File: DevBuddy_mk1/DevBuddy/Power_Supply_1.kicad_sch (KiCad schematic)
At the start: 1 part, among them U5 TPS54331DDAR

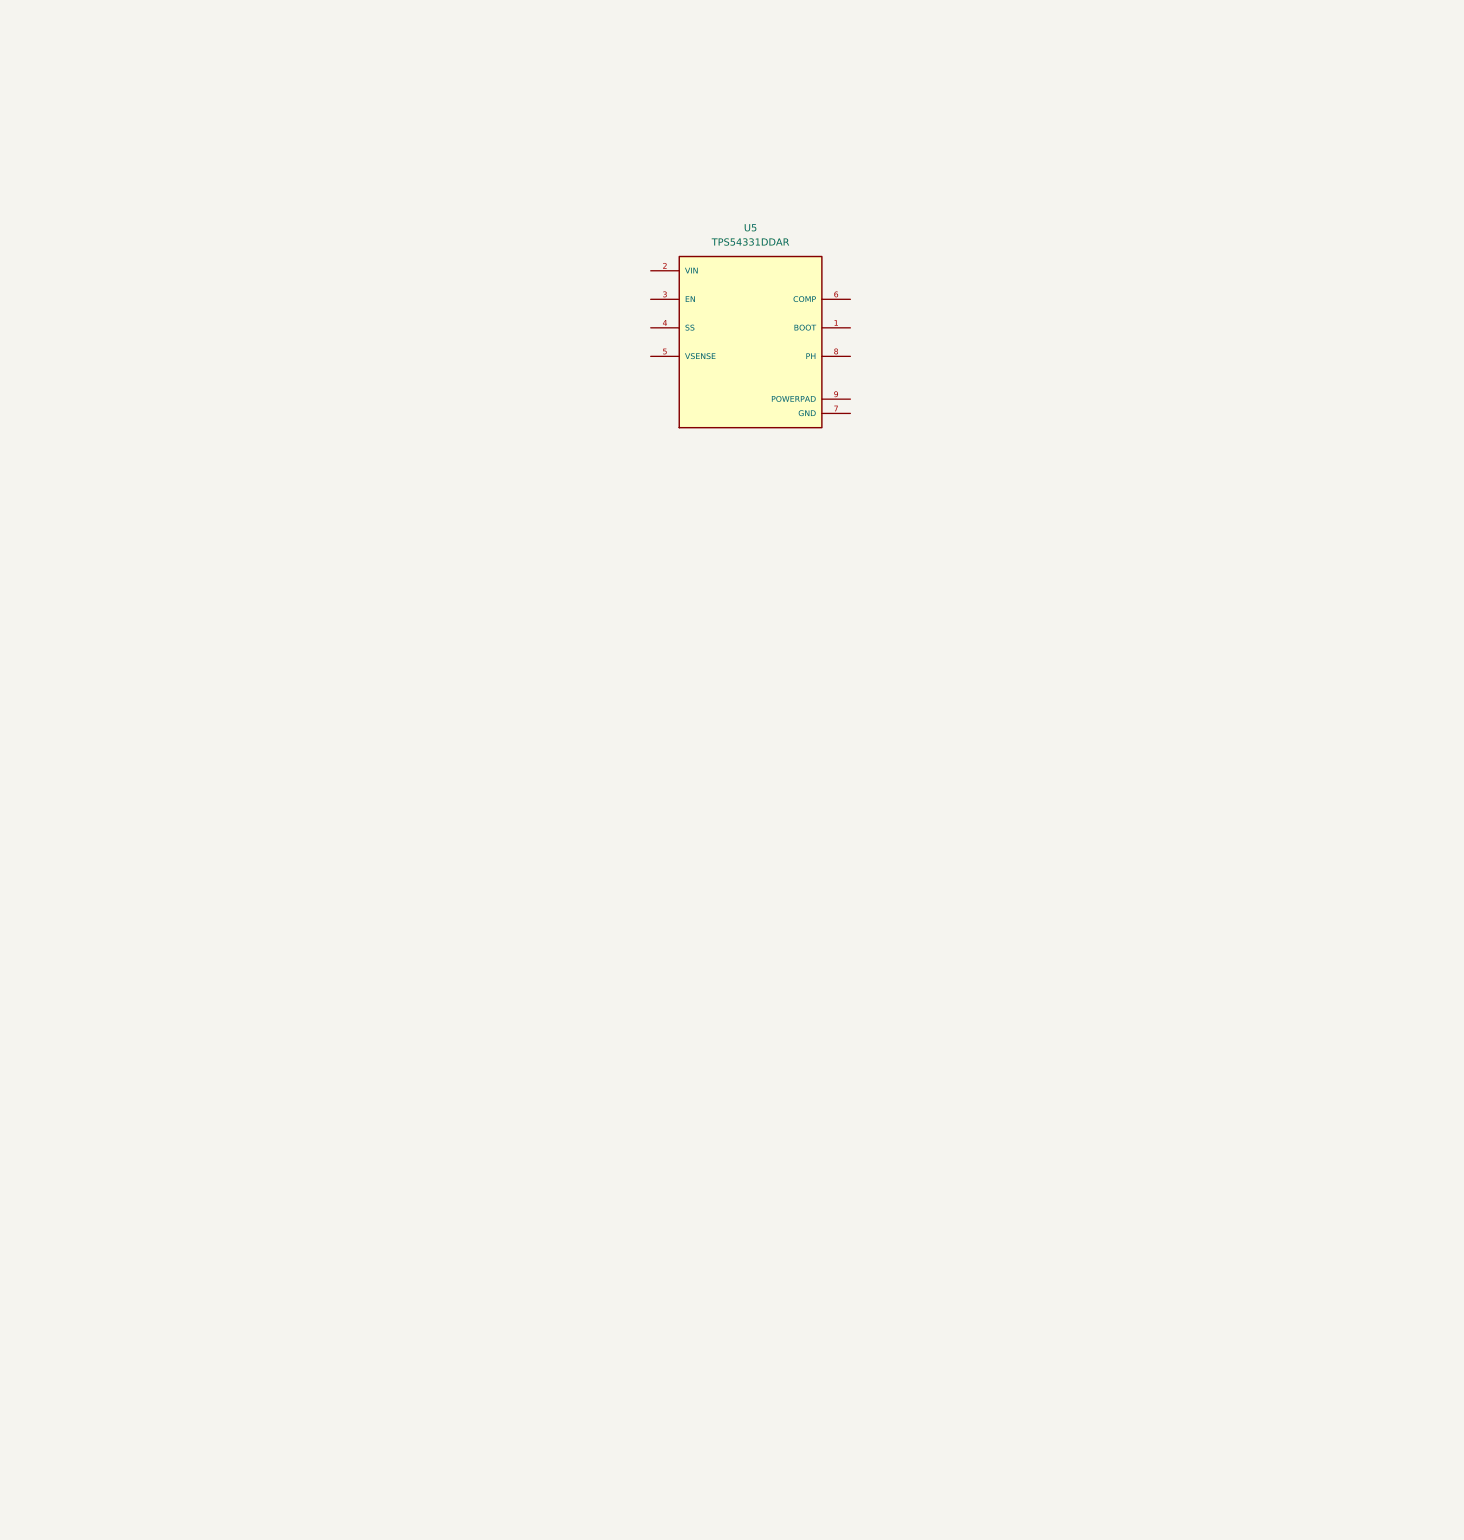
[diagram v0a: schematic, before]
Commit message: Changes is hardware - Power
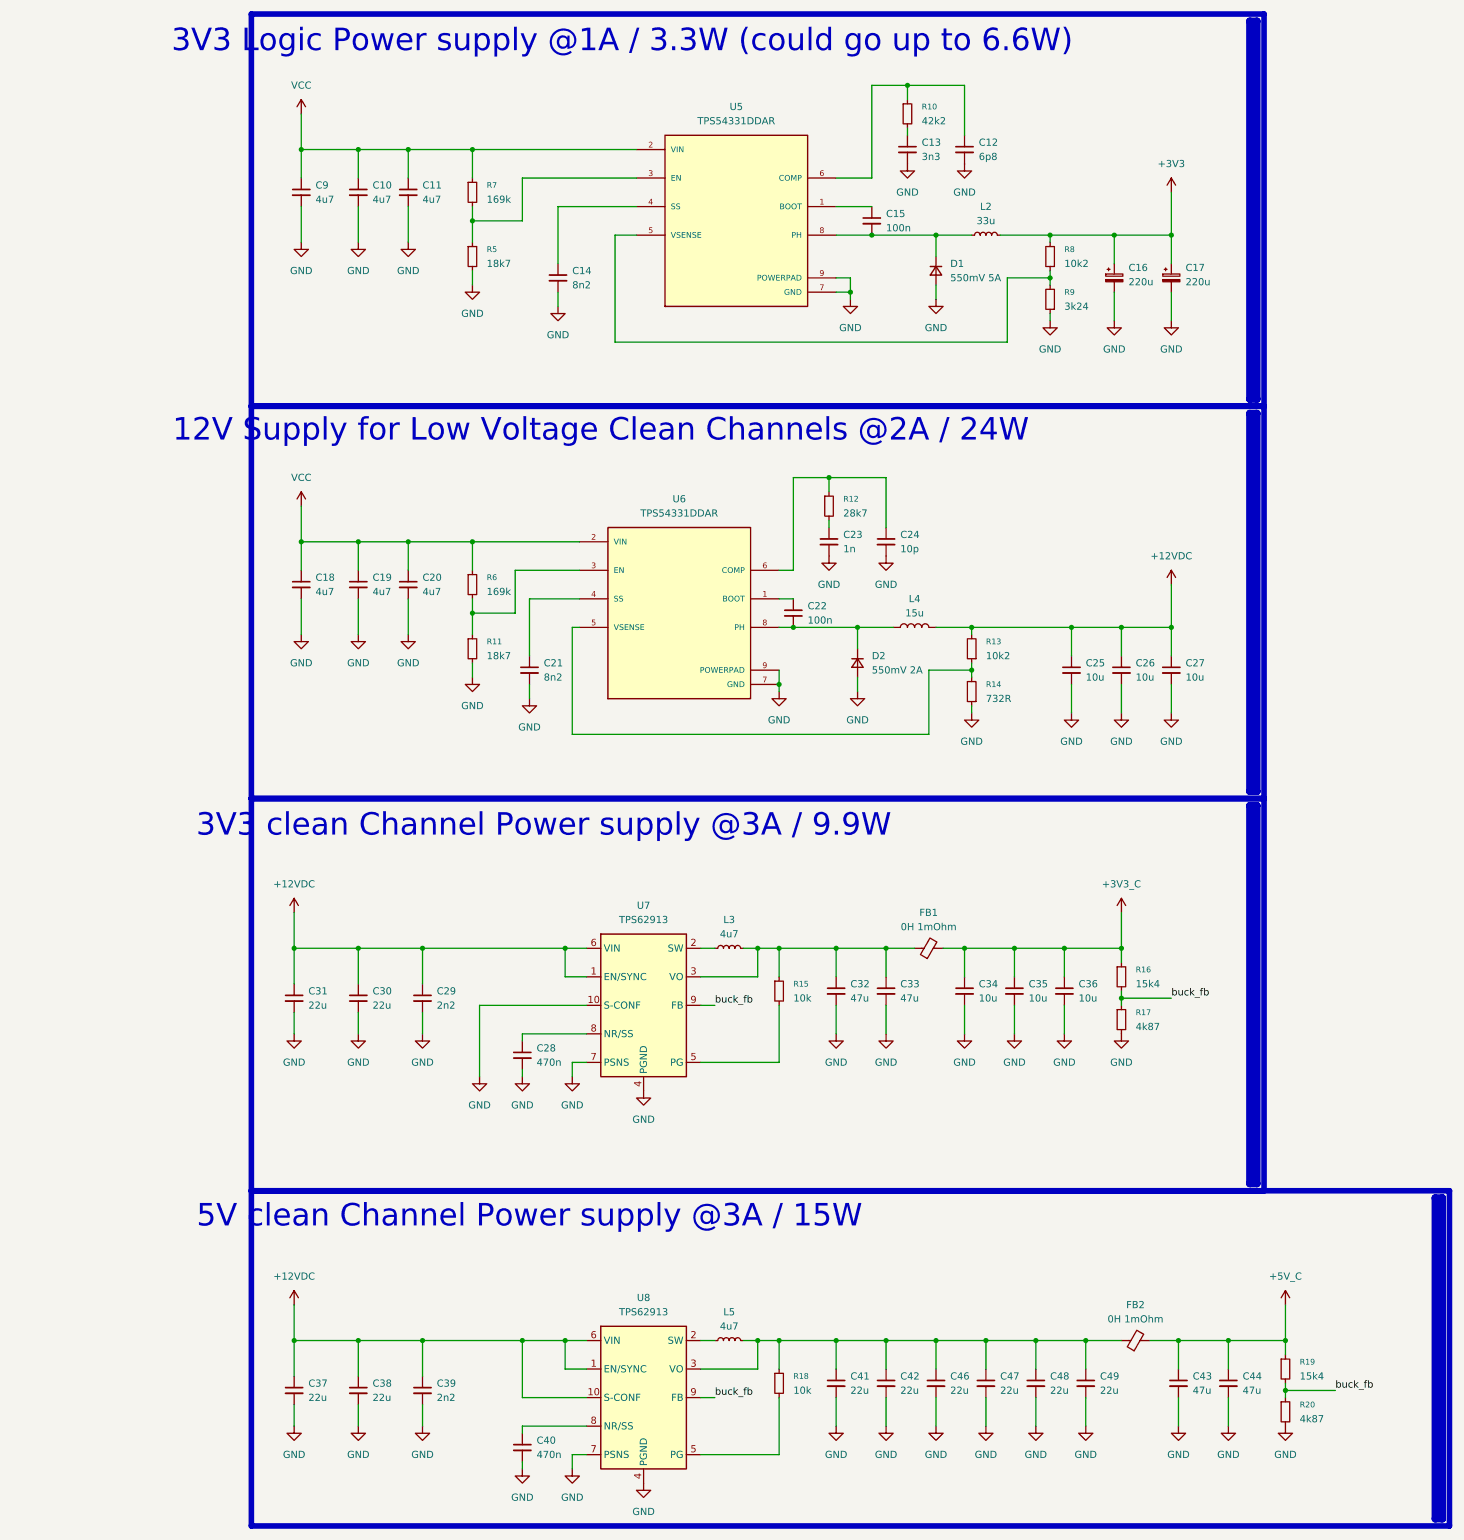
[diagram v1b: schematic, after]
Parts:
- added C10, C11, C18, C19, C20, C9: 4u7, Capacitor_SMD:C_1210_3225Metric, symbol Device:C_Small
- added C12: 6p8, Capacitor_SMD:C_0402_1005Metric, symbol Device:C_Small
- added C13: 3n3, Capacitor_SMD:C_0402_1005Metric, symbol Device:C_Small
- added C14, C21: 8n2, Capacitor_SMD:C_0402_1005Metric, symbol Device:C_Small
- added C15, C22: 100n, Capacitor_SMD:C_0805_2012Metric, symbol Device:C_Small
- added C16, C17: 220u, Capacitor_SMD:CP_Elec_6.3x5.4, symbol Device:C_Polarized_Small
- added C23: 1n, Capacitor_SMD:C_0402_1005Metric, symbol Device:C_Small
- added C24: 10p, Capacitor_SMD:C_0402_1005Metric, symbol Device:C_Small
- added C25, C26, C27: 10u, Capacitor_SMD:C_1210_3225Metric, symbol Device:C_Small
- added C28, C40: 470n, Capacitor_SMD:C_0402_1005Metric, symbol Device:C_Small
- added C29, C39: 2n2, Capacitor_SMD:C_0402_1005Metric, symbol Device:C_Small
- added C30, C31, C37, C38, C41, C42, C46, C47, C48, C49: 22u, Capacitor_SMD:C_0805_2012Metric, symbol Device:C_Small
- added C32, C33, C43, C44: 47u, Capacitor_SMD:C_0805_2012Metric, symbol Device:C_Small
- added C34, C35, C36: 10u, Capacitor_SMD:C_0805_2012Metric, symbol Device:C_Small
- added D1: 550mV 5A, Diode_SMD:D_SMC, symbol Device:D_Small
- added D2: 550mV 2A, Diode_SMD:D_SMC, symbol Device:D_Small
- added FB1, FB2: 0H 1mOhm, symbol Device:FerriteBead_Small
- added L2: 33u, Inductor_SMD:L_Coilcraft_MSS1210-XXX, symbol Device:L_Small
- added L3, L5: 4u7, Inductor_SMD:L_Coilcraft_XAL6060-XXX, symbol Device:L_Small
- added L4: 15u, Inductor_SMD:L_Bourns_SRR1260, symbol Device:L
- added R10: 42k2, Resistor_SMD:R_0402_1005Metric, symbol Device:R_Small
- added R11, R5: 18k7, Resistor_SMD:R_0402_1005Metric, symbol Device:R_Small
- added R12: 28k7, Resistor_SMD:R_0402_1005Metric, symbol Device:R_Small
- added R13, R8: 10k2, Resistor_SMD:R_01005_0402Metric, symbol Device:R_Small
- added R14: 732R, Resistor_SMD:R_01005_0402Metric, symbol Device:R_Small
- added R15, R18: 10k, Resistor_SMD:R_0402_1005Metric, symbol Device:R_Small
- added R16, R19: 15k4, Resistor_SMD:R_0402_1005Metric, symbol Device:R_Small
- added R17, R20: 4k87, Resistor_SMD:R_0402_1005Metric, symbol Device:R_Small
- added R6, R7: 169k, Resistor_SMD:R_0402_1005Metric, symbol Device:R_Small
- added R9: 3k24, Resistor_SMD:R_01005_0402Metric, symbol Device:R_Small
- added U6: TPS54331DDAR, TPS54331DDAR:CONV_TPS54331DDAR, symbol TPS54331DDAR:TPS54331DDAR
- added U7, U8: TPS62913, Package_DFN_QFN:Texas_RPU0010A_VQFN-HR-10_2x2mm_P0.5mm, symbol Regulator_Switching:TPS62913
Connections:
- net at U5.1 (BOOT): now also C15.1
- net VCC: now reaches U5.2 (VIN)
- net VCC: now also C10.1, C11.1, C18.1, C19.1, C20.1, C9.1, R6.1, R7.1, U6.2 (VIN)
- net at U5.3 (EN): now also R5.1, R7.2
- net at U5.4 (SS): now also C14.1
- net at U5.5 (VSENSE): now also R8.1, R9.2
- net at U5.6 (COMP): now also C12.1, R10.1
- net GND: now reaches U5.7 (GND)
- net GND: now also U5.9 (POWERPAD), C10.2, C11.2, C12.2, C13.2, C14.2, C16.2, C17.2, C18.2, C19.2, C20.2, C21.2, C23.2, C24.2, C25.2, C26.2, C27.2, C28.2, C29.2, C30.2, C31.2, C32.2, C33.2, C34.2, C35.2, C36.2, C37.2, C38.2, C39.2, C40.2, C41.2, C42.2, C43.2, C44.2, C46.2, C47.2, C48.2, C49.2, C9.2, D1.2 (A), D2.2 (A), R11.2, R14.1, R17.2, R20.2, R5.2, R9.1, U6.7 (GND), U6.9 (POWERPAD), U7.10 (S-CONF), U7.4 (PGND), U7.7 (PSNS), U8.4 (PGND), U8.7 (PSNS)
- net at U5.8 (PH): now also C15.2, D1.1 (K), L2.1
- new net: C41.1, C42.1, C46.1, C47.1, C48.1, C49.1, FB2.1, L5.2, R18.1, U8.3 (VO)
- new net: C13.1, R10.2
- new net: R18.2, U8.5 (PG)
- new net: L3.1, U7.2 (SW)
- new net: C32.1, C33.1, FB1.1, L3.2, R15.1, U7.3 (VO)
- new net: L5.1, U8.2 (SW)
- new net: C40.1, U8.8 (NR/SS)
- new net: R11.1, R6.2, U6.3 (EN)
- new net: R13.1, R14.2, U6.5 (VSENSE)
- new net: C22.1, U6.1 (BOOT)
- new net: C21.1, U6.4 (SS)
- new net: C24.1, R12.1, U6.6 (COMP)
- new net: C22.2, D2.1 (K), L4.1, U6.8 (PH)
- new net: R15.2, U7.5 (PG)
- new net: C28.1, U7.8 (NR/SS)
- new net: C23.1, R12.2
- new net +12VDC: C25.1, C26.1, C27.1, C29.1, C30.1, C31.1, C37.1, C38.1, C39.1, L4.2, R13.2, U7.1 (EN/SYNC), U7.6 (VIN), U8.1 (EN/SYNC), U8.10 (S-CONF), U8.6 (VIN)
- new net +3V3: C16.1, C17.1, L2.2, R8.2
- new net +3V3_C: C34.1, C35.1, C36.1, FB1.2, R16.1
- new net +5V_C: C43.1, C44.1, FB2.2, R19.1
- new net buck_fb: R16.2, R17.1, R19.2, R20.1, U7.9 (FB), U8.9 (FB)
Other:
- note added: "12V Supply for Low Voltage Clean Channels @2A / 24W"
- note added: "3V3 Logic Power supply @1A / 3.3W (could go up to 6.6W)"
- note added: "3V3 clean Channel Power supply @3A / 9.9W"
- note added: "5V clean Channel Power supply @3A / 15W"
- moved on the sheet: U5
